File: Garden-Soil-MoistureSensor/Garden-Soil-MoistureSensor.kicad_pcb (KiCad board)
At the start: 2 copper layers, 68.6 x 92.8 mm, 11 parts, among them IC1 CD74HC4067M96, IC2 CD74HC4067M96, J1 Conn_01x15, J2 Conn_01x15, J3 Conn_02x15_Odd_Even, U1 1043

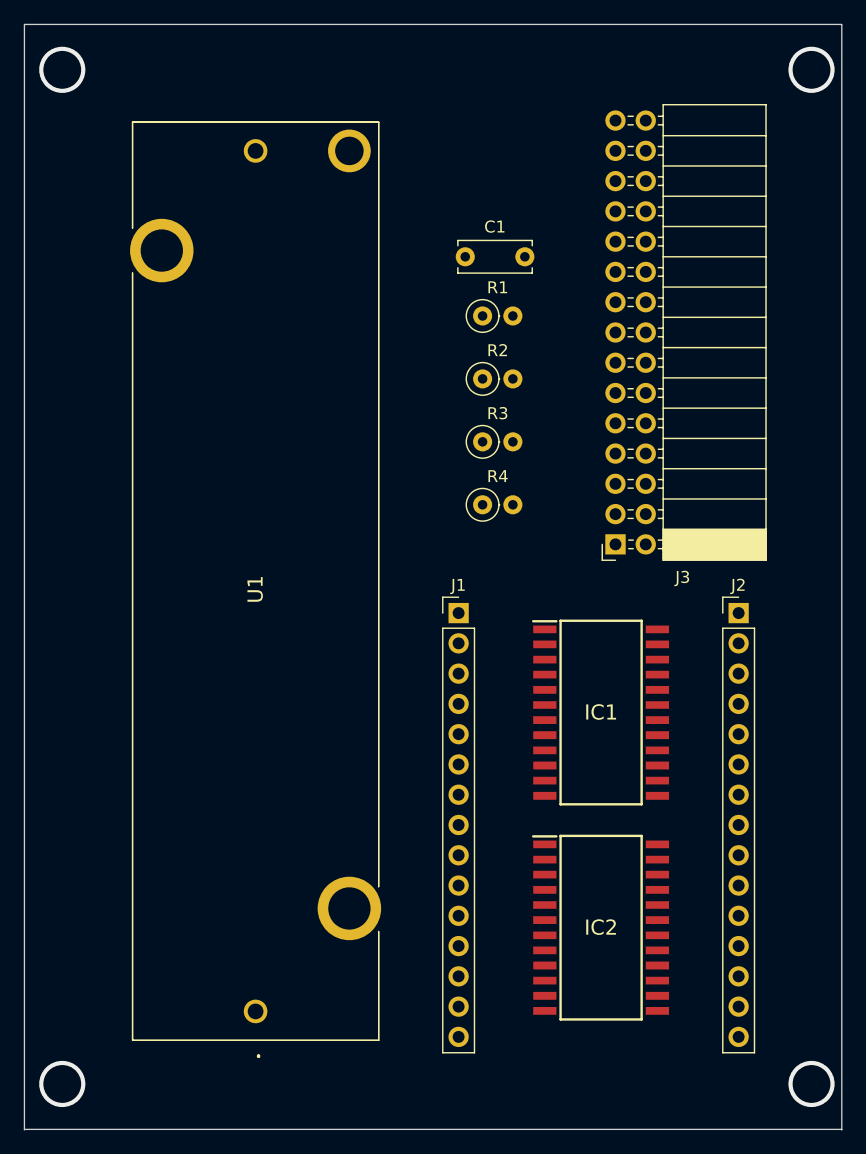
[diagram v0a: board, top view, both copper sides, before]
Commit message: drc fixes pre route
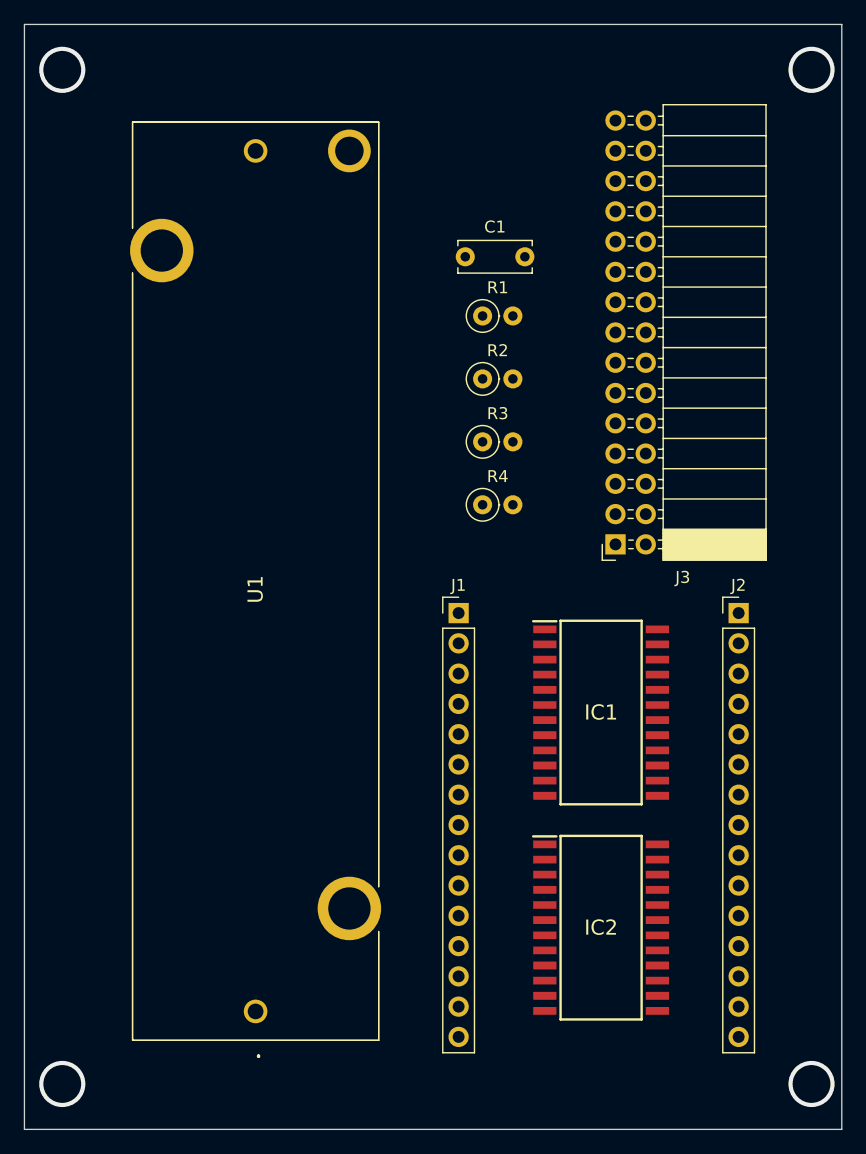
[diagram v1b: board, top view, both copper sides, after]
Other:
- board size 68.6 x 92.8 mm -> 68.6 x 92.7 mm
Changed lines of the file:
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@@
     )
   )
-  (gr_line (start 114.3 45.72) (end 114.3 138.475913) (layer "Edge.Cuts") (width 0.1))
+  (gr_line (start 114.3 45.72) (end 114.3 138.43) (layer "Edge.Cuts") (width 0.1))
   (gr_line (start 182.88 45.72) (end 114.3 45.72) (layer "Edge.Cuts") (width 0.1))
   (gr_line (start 114.3 138.43) (end 182.88 138.43) (layer "Edge.Cuts") (width 0.1))
-  (gr_line (start 182.88 138.48139) (end 182.88 45.754492) (layer "Edge.Cuts") (width 0.1))
+  (gr_line (start 182.88 138.43) (end 182.88 45.72) (layer "Edge.Cuts") (width 0.1))
   (via (at 117.475 49.53) (size 3.8736) (drill 3.175) (layers "F.Cu" "B.Cu") (free) (net 10))
   (via (at 117.475 134.62) (size 3.8736) (drill 3.175) (layers "F.Cu" "B.Cu") (free) (net 10))
